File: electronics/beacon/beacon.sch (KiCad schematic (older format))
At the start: 15 parts, among them J1 CONN_01X01, J2 CONN_01X01, J3 CONN_02X04, Q1 Q_NMOS_GSD, U1 ATTINY45-20XUR, U2 TPS70928DBV

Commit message: Finalize beacon schematic for initial run
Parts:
- removed J3: CONN_02X04, symbol CONN_02X04
- C1: value 1uF -> 1u
- C2: value 22uF -> 22u
- J1: value CONN_01X01 -> RAIL1
- J2: value CONN_01X01 -> RAIL2
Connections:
- net labels removed: Rail1, Rail2, VCC
- wire segments 48 -> 39
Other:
- note added: "Control"
- note added: "IR LED"
- note added: "Power"
- moved on the sheet: C1, C2, D1, D2, J1, J2, Q1, R1, R2, R3, R4, R5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

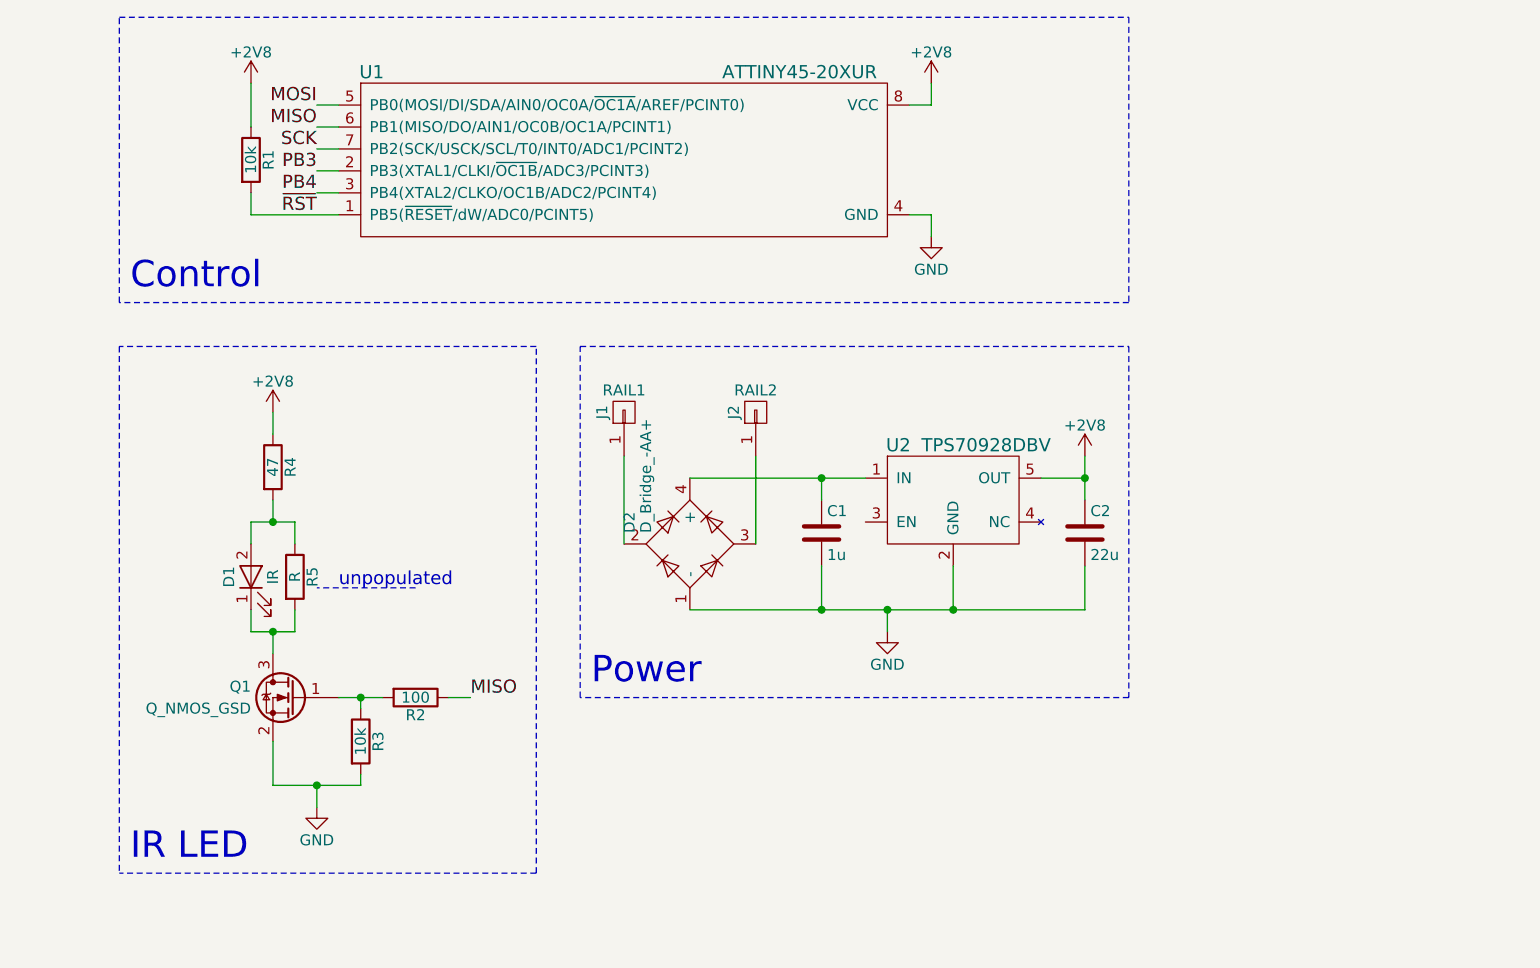
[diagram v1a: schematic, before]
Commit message: electronics: beacon: WIP 3.5x28 board layout
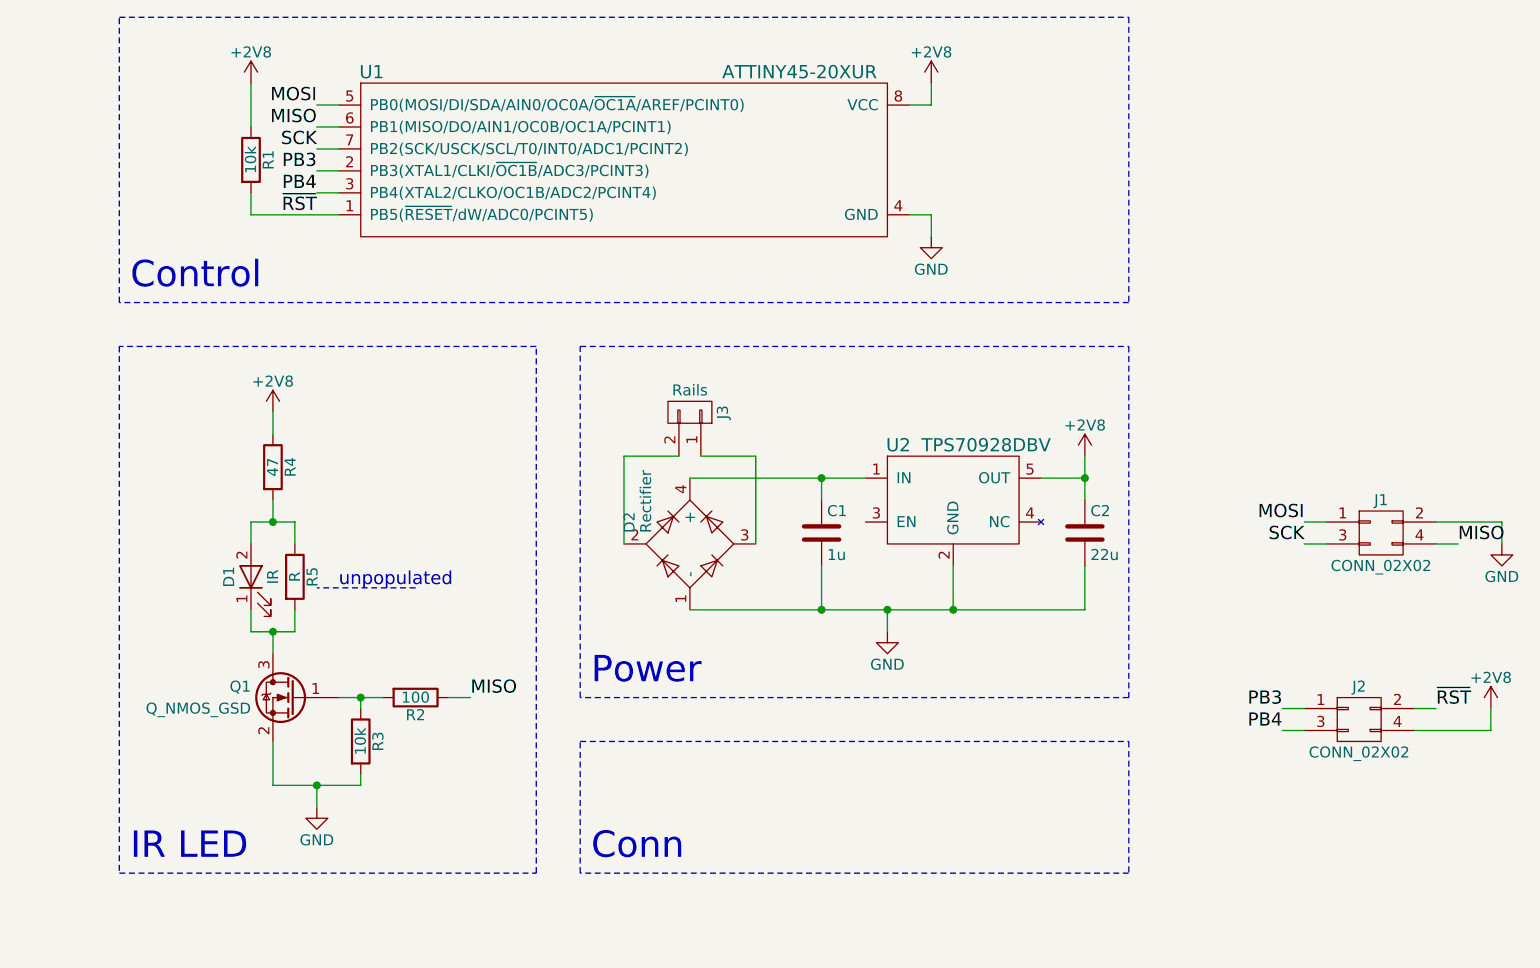
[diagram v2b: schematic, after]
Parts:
- removed J1: RAIL1, symbol CONN_01X01
- removed J2: RAIL2, symbol CONN_01X01
- added J1, J2: CONN_02X02, bcan:Edge_Connector_2x02_Pitch2.54mm_SMD, symbol CONN_02X02
- added J3: Rails, bcan:HO_Rail_2_Length3.5mm_Width3mm, symbol CONN_01X02
- C1, C2: footprint Capacitors_SMD:C_0603_HandSoldering -> Capacitors_SMD:C_0603
- D2: value D_Bridge_-AA+ -> Rectifier
- R1, R2, R3, R4, R5: footprint Resistors_SMD:R_0603_HandSoldering -> Resistors_SMD:R_0603
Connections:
- net +2V8: now also J2.4 (P4)
- net GND: now also J1.2 (P2)
- net MISO: now also J1.4 (P4)
- net MOSI: now also J1.1 (P1)
- net PB3: now also J2.1 (P1)
- net PB4: now also J2.3 (P3)
- net SCK: now also J1.3 (P3)
- net ~RST: now also J2.2 (P2)
- net at D2.2: now also J3.2 (P2)
- net at D2.3: now also J3.1 (P1)
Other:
- note added: "Conn"
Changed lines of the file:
@@
 P 6200 4700
 F 0 "D2" H 6250 4975 50  0000 L CNN
-F 1 "D_Bridge_-AA+" H 6250 4900 50  0000 L CNN
+F 1 "Rectifier" H 6250 4900 50  0000 L CNN
 F 2 "TO_SOT_Packages_SMD:SOT-143" H 6200 4700 50  0001 C CNN
 F 3 "" H 6200 4700 50  0000 C CNN
@@
 F 0 "C1" H 6825 4750 50  0000 L CNN
 F 1 "1u" H 6825 4550 50  0000 L CNN
-F 2 "Capacitors_SMD:C_0603_HandSoldering" H 6838 4500 50  0001 C CNN
+F 2 "Capacitors_SMD:C_0603" H 6838 4500 50  0001 C CNN
 F 3 "" H 6800 4650 50  0000 C CNN
 	1    6800 4650
@@
 F 0 "R2" V 5030 5400 50  0000 C CNN
 F 1 "100" V 4950 5400 50  0000 C CNN
-F 2 "Resistors_SMD:R_0603_HandSoldering" V 4880 5400 50  0001 C CNN
+F 2 "Resistors_SMD:R_0603" V 4880 5400 50  0001 C CNN
 F 3 "" H 4950 5400 50  0000 C CNN
 	1    4950 5400
@@
 F 0 "R4" V 4380 4350 50  0000 C CNN
 F 1 "47" V 4300 4350 50  0000 C CNN
-F 2 "Resistors_SMD:R_0603_HandSoldering" V 4230 4350 50  0001 C CNN
+F 2 "Resistors_SMD:R_0603" V 4230 4350 50  0001 C CNN
 F 3 "" H 4300 4350 50  0000 C CNN
 	1    4300 4350
@@
 F 0 "R1" V 4280 2950 50  0000 C CNN
 F 1 "10k" V 4200 2950 50  0000 C CNN
-F 2 "Resistors_SMD:R_0603_HandSoldering" V 4130 2950 50  0001 C CNN
+F 2 "Resistors_SMD:R_0603" V 4130 2950 50  0001 C CNN
 F 3 "" H 4200 2950 50  0000 C CNN
 	1    4200 2950
@@
 F 0 "R3" V 4780 5600 50  0000 C CNN
 F 1 "10k" V 4700 5600 50  0000 C CNN
-F 2 "Resistors_SMD:R_0603_HandSoldering" V 4630 5600 50  0001 C CNN
+F 2 "Resistors_SMD:R_0603" V 4630 5600 50  0001 C CNN
 F 3 "" H 4700 5600 50  0001 C CNN
 	1    4700 5600
@@
 F 0 "C2" H 8025 4750 50  0000 L CNN
 F 1 "22u" H 8025 4550 50  0000 L CNN
-F 2 "Capacitors_SMD:C_0603_HandSoldering" H 8038 4500 50  0001 C CNN
+F 2 "Capacitors_SMD:C_0603" H 8038 4500 50  0001 C CNN
 F 3 "" H 8000 4650 50  0001 C CNN
 	1    8000 4650
@@
 F 0 "R5" V 4480 4850 50  0000 C CNN
 F 1 "R" V 4400 4850 50  0000 C CNN
-F 2 "Resistors_SMD:R_0603_HandSoldering" V 4330 4850 50  0001 C CNN
+F 2 "Resistors_SMD:R_0603" V 4330 4850 50  0001 C CNN
 F 3 "" H 4400 4850 50  0000 C CNN
 	1    4400 4850
 	1    0    0    -1
-$EndComp
-$Comp
-L CONN_01X01 J1
-U 1 1 58ABA652
-P 5900 4100
-F 0 "J1" H 5900 4200 50  0000 C CNN
-F 1 "RAIL1" V 6000 4100 50  0000 C CNN
-F 2 "" H 5900 4100 50  0001 C CNN
-F 3 "" H 5900 4100 50  0001 C CNN
-	1    5900 4100
-	0    -1   -1   0
-$EndComp
-$Comp
-L CONN_01X01 J2
-U 1 1 58ABA785
-P 6500 4100
-F 0 "J2" H 6500 4200 50  0000 C CNN
-F 1 "RAIL2" V 6600 4100 50  0000 C CNN
-F 2 "" H 6500 4100 50  0001 C CNN
-F 3 "" H 6500 4100 50  0001 C CNN
-	1    6500 4100
-	0    -1   -1   0
 $EndComp
 Text Label 5200 5400 0    60   ~ 0
@@
 Text Notes 3650 6150 0    120  ~ 0
 IR LED
-Wire Wire Line
-	7800 4400 8000 4400
-Wire Notes Line
-	4950 4900 4500 4900
-Wire Wire Line
-	7300 2700 7300 2600
-Wire Wire Line
-	7200 2700 7300 2700
-Wire Wire Line
-	6500 4700 6500 4300
-Wire Wire Line
-	5900 4700 5900 4300
-Connection ~ 8000 4400
-Wire Wire Line
-	8000 4300 8000 4500
-Connection ~ 4700 5400
-Connection ~ 4500 5800
-Wire Wire Line
-	4300 5600 4300 5800
-Wire Wire Line
-	4500 5800 4500 5900
-Wire Wire Line
-	4300 5800 4700 5800
-Wire Wire Line
-	4700 5800 4700 5750
-Wire Wire Line
-	4700 5400 4700 5450
-Wire Wire Line
-	4600 5400 4800 5400
-Wire Wire Line
-	4200 2800 4200 2600
-Wire Wire Line
-	4200 3200 4200 3100
-Wire Wire Line
-	4200 3200 4600 3200
-Connection ~ 4300 5100
-Wire Wire Line
-	4300 5100 4300 5200
-Wire Wire Line
-	4200 5100 4400 5100
-Wire Wire Line
-	4300 4200 4300 4100
-Connection ~ 4300 4600
-Wire Wire Line
-	4300 4600 4300 4500
-Wire Wire Line
-	4400 4600 4400 4700
-Wire Wire Line
-	4200 4600 4400 4600
-Wire Wire Line
-	4200 4700 4200 4600
-Wire Wire Line
-	4400 5100 4400 5000
-Wire Wire Line
-	4200 5000 4200 5100
-Wire Wire Line
-	8000 5000 8000 4800
-Connection ~ 6800 5000
-Wire Wire Line
-	6800 5000 6800 4800
-Wire Wire Line
-	7200 3200 7300 3200
-Wire Wire Line
-	7300 3200 7300 3300
-Wire Wire Line
-	7100 5000 7100 5100
-Connection ~ 7100 5000
-Wire Wire Line
-	7400 5000 7400 4800
-Connection ~ 7400 5000
-Wire Wire Line
-	6200 5000 8000 5000
-Wire Wire Line
-	5100 5400 5200 5400
-Wire Notes Line
-	5500 6200 3600 6200
-Wire Notes Line
-	3600 3600 3600 2300
-Wire Notes Line
-	8200 2300 8200 3600
-Wire Notes Line
-	5700 5400 5700 3800
-Wire Notes Line
-	5700 3800 8200 3800
-Wire Notes Line
-	8200 3800 8200 5400
-Wire Notes Line
-	8200 5400 5700 5400
-Wire Notes Line
-	5500 6200 5500 3800
-Wire Notes Line
-	5500 3800 3600 3800
-Wire Notes Line
-	3600 3800 3600 6200
-Wire Notes Line
-	3600 2300 8200 2300
-Wire Notes Line
-	8200 3600 3600 3600
-Wire Wire Line
-	4600 2700 4500 2700
-Wire Wire Line
-	4600 2800 4500 2800
-Wire Wire Line
-	4600 2900 4500 2900
 Text Label 4500 2700 2    60   ~ 0
 MOSI
@@
 Text Label 4500 2900 2    60   ~ 0
 SCK
-Wire Wire Line
-	4600 3100 4500 3100
-Wire Wire Line
-	4600 3000 4500 3000
 Text Label 4500 3000 2    60   ~ 0
 PB3
 Text Label 4500 3100 2    60   ~ 0
 PB4
+$Comp
+L CONN_01X02 J3
+U 1 1 58C5B8EB
+P 6200 4100
+F 0 "J3" H 6200 4250 50  0000 C CNN
+F 1 "Rails" V 6300 4100 50  0000 C CNN
+F 2 "bcan:HO_Rail_2_Length3.5mm_Width3mm" H 6200 4100 50  0001 C CNN
+F 3 "" H 6200 4100 50  0001 C CNN
+	1    6200 4100
+	0    1    -1   0
+$EndComp
+Text Notes 5750 6150 0    120  ~ 0
+Conn
+$Comp
+L CONN_02X02 J1
+U 1 1 58C61A56
+P 9350 4650
+F 0 "J1" H 9350 4800 50  0000 C CNN
+F 1 "CONN_02X02" H 9350 4500 50  0000 C CNN
+F 2 "bcan:Edge_Connector_2x02_Pitch2.54mm_SMD" H 9350 3450 50  0001 C CNN
+F 3 "" H 9350 3450 50  0001 C CNN
+	1    9350 4650
+	1    0    0    -1
+$EndComp
+$Comp
+L CONN_02X02 J2
+U 1 1 58C61B0B
+P 9250 5500
+F 0 "J2" H 9250 5650 50  0000 C CNN
+F 1 "CONN_02X02" H 9250 5350 50  0000 C CNN
+F 2 "bcan:Edge_Connector_2x02_Pitch2.54mm_SMD" H 9250 4300 50  0001 C CNN
+F 3 "" H 9250 4300 50  0001 C CNN
+	1    9250 5500
+	1    0    0    -1
+$EndComp
+Text Label 9000 4600 2    60   ~ 0
+MOSI
+Text Label 9000 4700 2    60   ~ 0
+SCK
+$Comp
+L +2V8 #PWR08
+U 1 1 58C62508
+P 9850 5450
+F 0 "#PWR08" H 9850 5300 50  0001 C CNN
+F 1 "+2V8" H 9850 5590 50  0000 C CNN
+F 2 "" H 9850 5450 50  0001 C CNN
+F 3 "" H 9850 5450 50  0001 C CNN
+	1    9850 5450
+	1    0    0    -1
+$EndComp
+Wire Wire Line
+	9100 4700 9000 4700
+Wire Wire Line
+	9100 4600 9000 4600
+Wire Wire Line
+	9000 5550 8900 5550
+Wire Wire Line
+	9000 5450 8900 5450
+Wire Wire Line
+	9500 5450 9600 5450
+Wire Notes Line
+	5700 6200 5700 5600
+Wire Notes Line
+	8200 6200 5700 6200
+Wire Notes Line
+	8200 5600 8200 6200
+Wire Notes Line
+	5700 5600 8200 5600
+Wire Wire Line
+	7800 4400 8000 4400
+Wire Notes Line
+	4950 4900 4500 4900
+Wire Wire Line
+	7300 2700 7300 2600
+Wire Wire Line
+	7200 2700 7300 2700
+Connection ~ 8000 4400
+Wire Wire Line
+	8000 4300 8000 4500
+Connection ~ 4700 5400
+Connection ~ 4500 5800
+Wire Wire Line
+	4300 5600 4300 5800
+Wire Wire Line
+	4500 5800 4500 5900
+Wire Wire Line
+	4300 5800 4700 5800
+Wire Wire Line
+	4700 5800 4700 5750
+Wire Wire Line
+	4700 5400 4700 5450
+Wire Wire Line
+	4600 5400 4800 5400
+Wire Wire Line
+	4200 2800 4200 2600
+Wire Wire Line
+	4200 3200 4200 3100
+Wire Wire Line
+	4200 3200 4600 3200
+Connection ~ 4300 5100
+Wire Wire Line
+	4300 5100 4300 5200
+Wire Wire Line
+	4200 5100 4400 5100
+Wire Wire Line
+	4300 4200 4300 4100
+Connection ~ 4300 4600
+Wire Wire Line
+	4300 4600 4300 4500
+Wire Wire Line
+	4400 4600 4400 4700
+Wire Wire Line
+	4200 4600 4400 4600
+Wire Wire Line
+	4200 4700 4200 4600
+Wire Wire Line
+	4400 5100 4400 5000
+Wire Wire Line
+	4200 5000 4200 5100
+Wire Wire Line
+	8000 5000 8000 4800
+Connection ~ 6800 5000
+Wire Wire Line
+	6800 5000 6800 4800
+Wire Wire Line
+	7200 3200 7300 3200
+Wire Wire Line
+	7300 3200 7300 3300
+Wire Wire Line
+	7100 5000 7100 5100
+Connection ~ 7100 5000
+Wire Wire Line
+	7400 5000 7400 4800
+Connection ~ 7400 5000
+Wire Wire Line
+	6200 5000 8000 5000
+Wire Wire Line
+	5100 5400 5200 5400
+Wire Notes Line
+	3600 6200 5500 6200
+Wire Notes Line
+	3600 3600 3600 2300
+Wire Notes Line
+	8200 2300 8200 3600
+Wire Notes Line
+	5700 5400 5700 3800
+Wire Notes Line
+	5700 3800 8200 3800
+Wire Notes Line
+	8200 3800 8200 5400
+Wire Notes Line
+	8200 5400 5700 5400
+Wire Notes Line
+	5500 6200 5500 3800
+Wire Notes Line
+	5500 3800 3600 3800
+Wire Notes Line
+	3600 3800 3600 6200
+Wire Notes Line
+	3600 2300 8200 2300
+Wire Notes Line
+	8200 3600 3600 3600
+Wire Wire Line
+	4600 2700 4500 2700
+Wire Wire Line
+	4600 2800 4500 2800
+Wire Wire Line
+	4600 2900 4500 2900
+Wire Wire Line
+	4600 3100 4500 3100
+Wire Wire Line
+	4600 3000 4500 3000
 Wire Wire Line
 	6200 4400 7000 4400
@@
 	6800 4500 6800 4400
 Connection ~ 6800 4400
+Wire Wire Line
+	6150 4300 5900 4300
+Wire Wire Line
+	5900 4300 5900 4700
+Wire Wire Line
+	6250 4300 6500 4300
+Wire Wire Line
+	6500 4300 6500 4700
+Text Label 9600 5450 0    60   ~ 0
+~RST
+Text Label 8900 5450 2    60   ~ 0
+PB3
+Text Label 8900 5550 2    60   ~ 0
+PB4
+Wire Wire Line
+	9500 5550 9850 5550
+Wire Wire Line
+	9850 5550 9850 5450
+$Comp
+L GND #PWR09
+U 1 1 58C62B36
+P 9900 4700
+F 0 "#PWR09" H 9900 4450 50  0001 C CNN
+F 1 "GND" H 9900 4550 50  0000 C CNN
+F 2 "" H 9900 4700 50  0001 C CNN
+F 3 "" H 9900 4700 50  0001 C CNN
+	1    9900 4700
+	1    0    0    -1
+$EndComp
+Wire Wire Line
+	9600 4600 9900 4600
+Wire Wire Line
+	9900 4600 9900 4700
+Wire Wire Line
+	9600 4700 9700 4700
+Text Label 9700 4700 0    60   ~ 0
+MISO
 $EndSCHEMATC
